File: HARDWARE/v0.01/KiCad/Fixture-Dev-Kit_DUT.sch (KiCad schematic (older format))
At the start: 33 parts, among them J62 Conn_01x20, J63 Conn_01x20, J64 Conn_01x20, J65 Conn_01x20, J66 CHIP4RH, J67 CHIP4LH, J68 Conn_01x35, J69 CHIP4B2B, J70 VBUS, J71 A_D+, J72 USB_OTG, J73 B_D-, J74 USB_A, J75 B_D+, J76 A_D-, J77 USB_ID, J78 Conn_01x35, J79 BAT, J80 UPDATE, J81 D-TP's, J82 ANT--SELECT, SW10 SW_Push

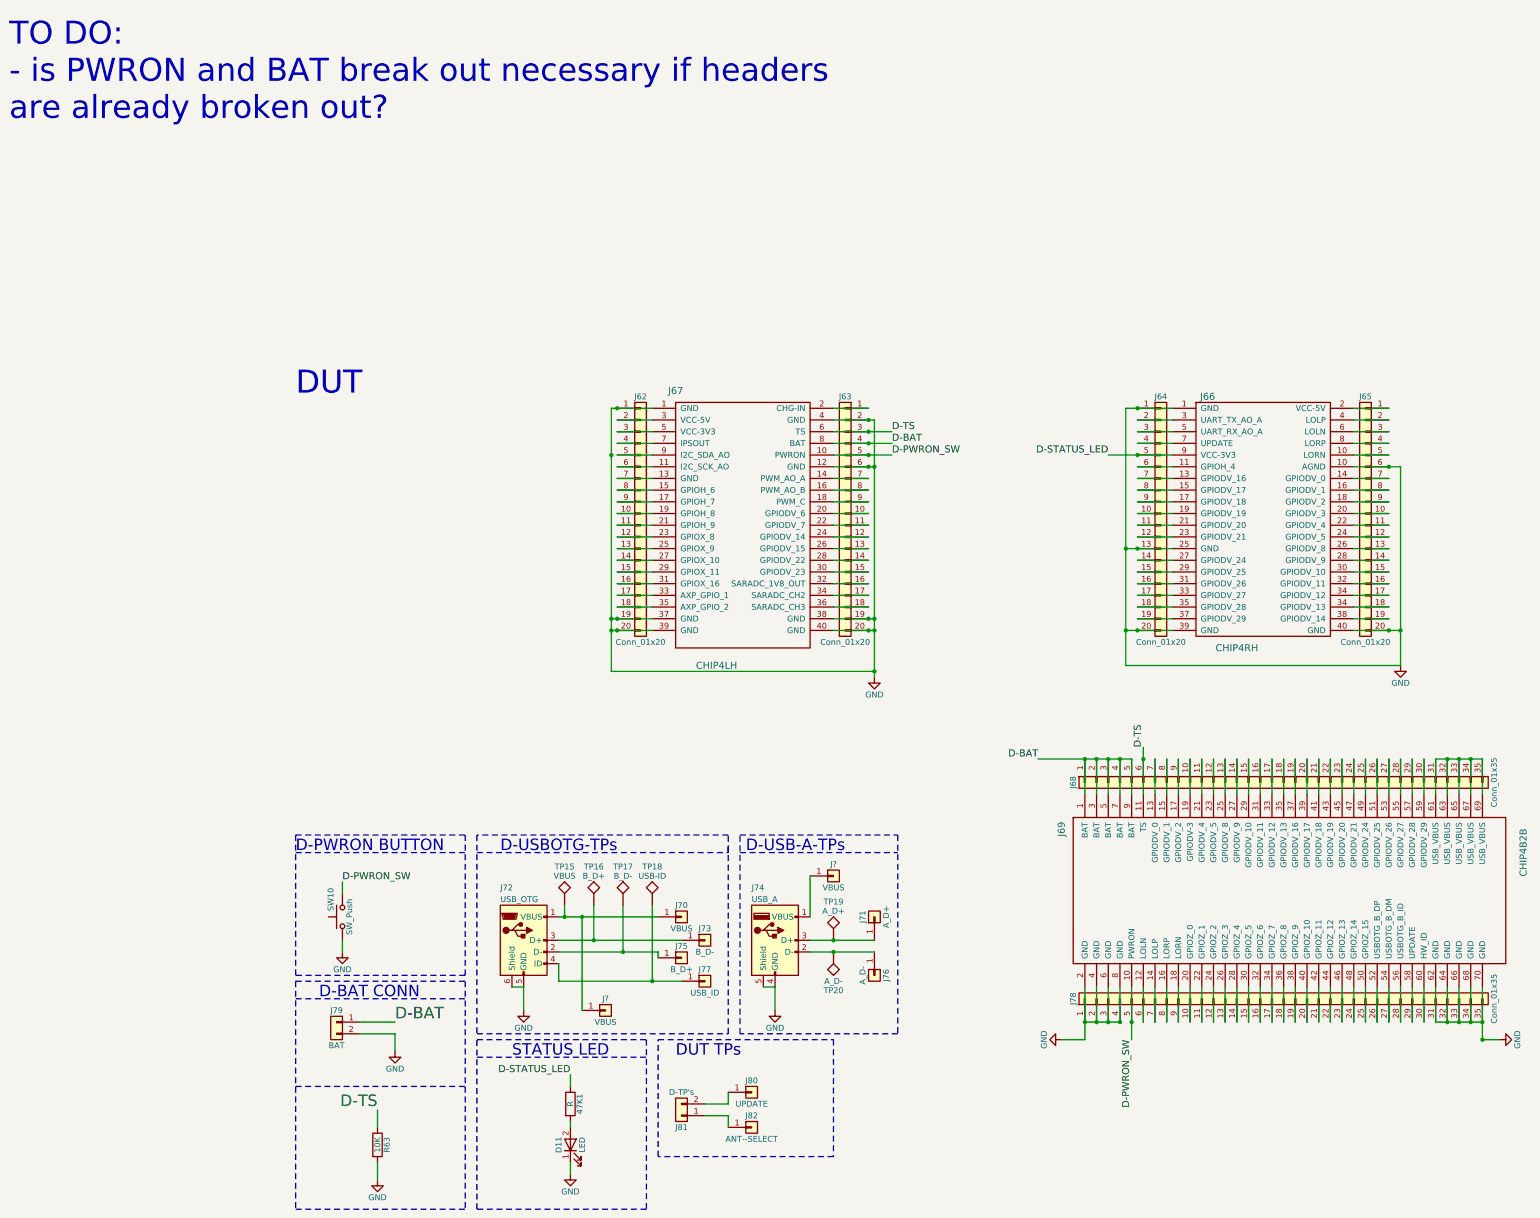
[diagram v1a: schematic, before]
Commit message: updating the cover page
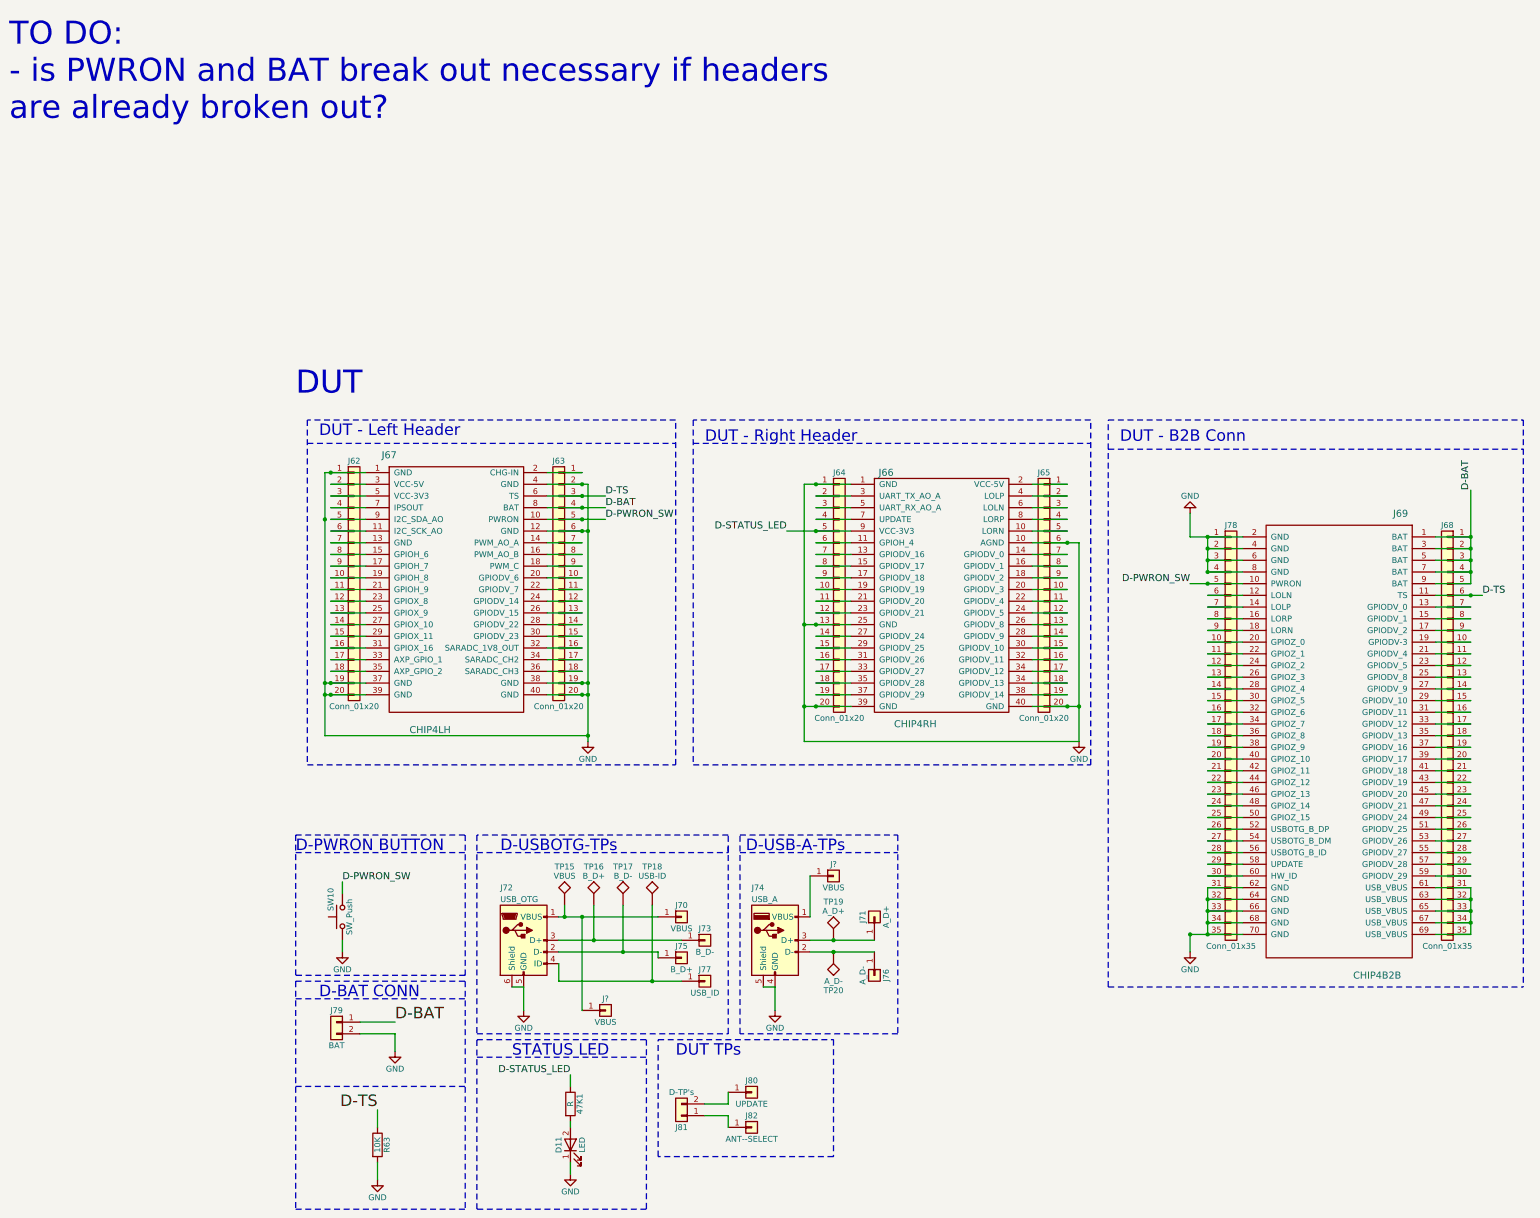
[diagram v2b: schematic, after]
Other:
- note added: "DUT - B2B Conn"
- note added: "DUT - Left Header"
- note added: "DUT - Right Header"
- moved on the sheet: J62, J63, J64, J65, J66, J67, J68, J69, J78
